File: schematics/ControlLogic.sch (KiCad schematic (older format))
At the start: 22 parts

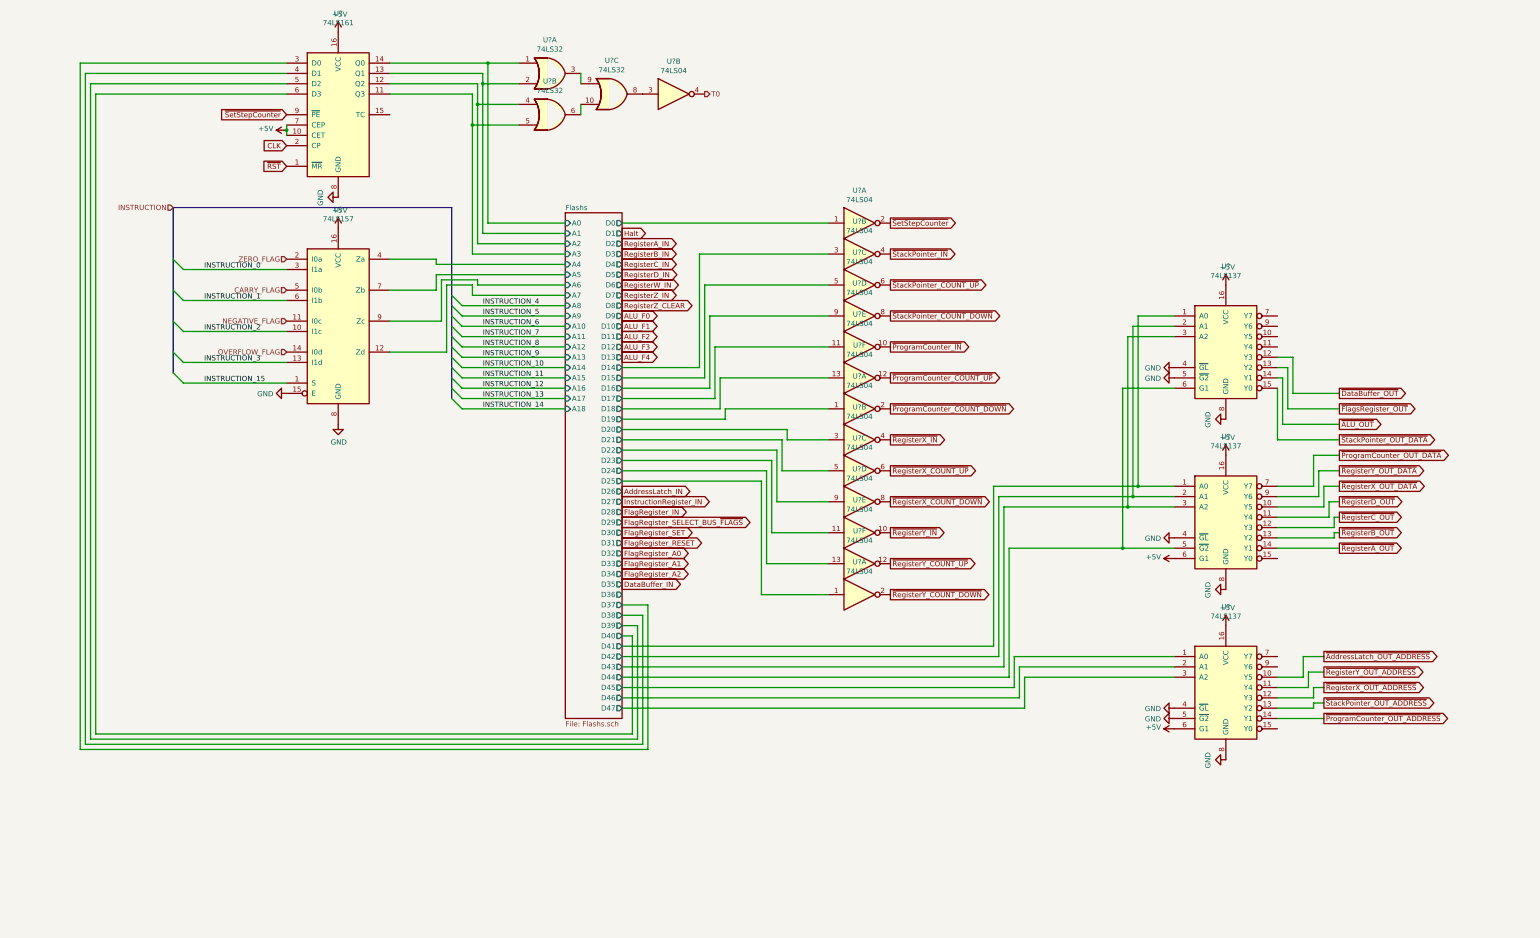
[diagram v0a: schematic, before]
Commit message: rearrange outputs of microcode eeproms
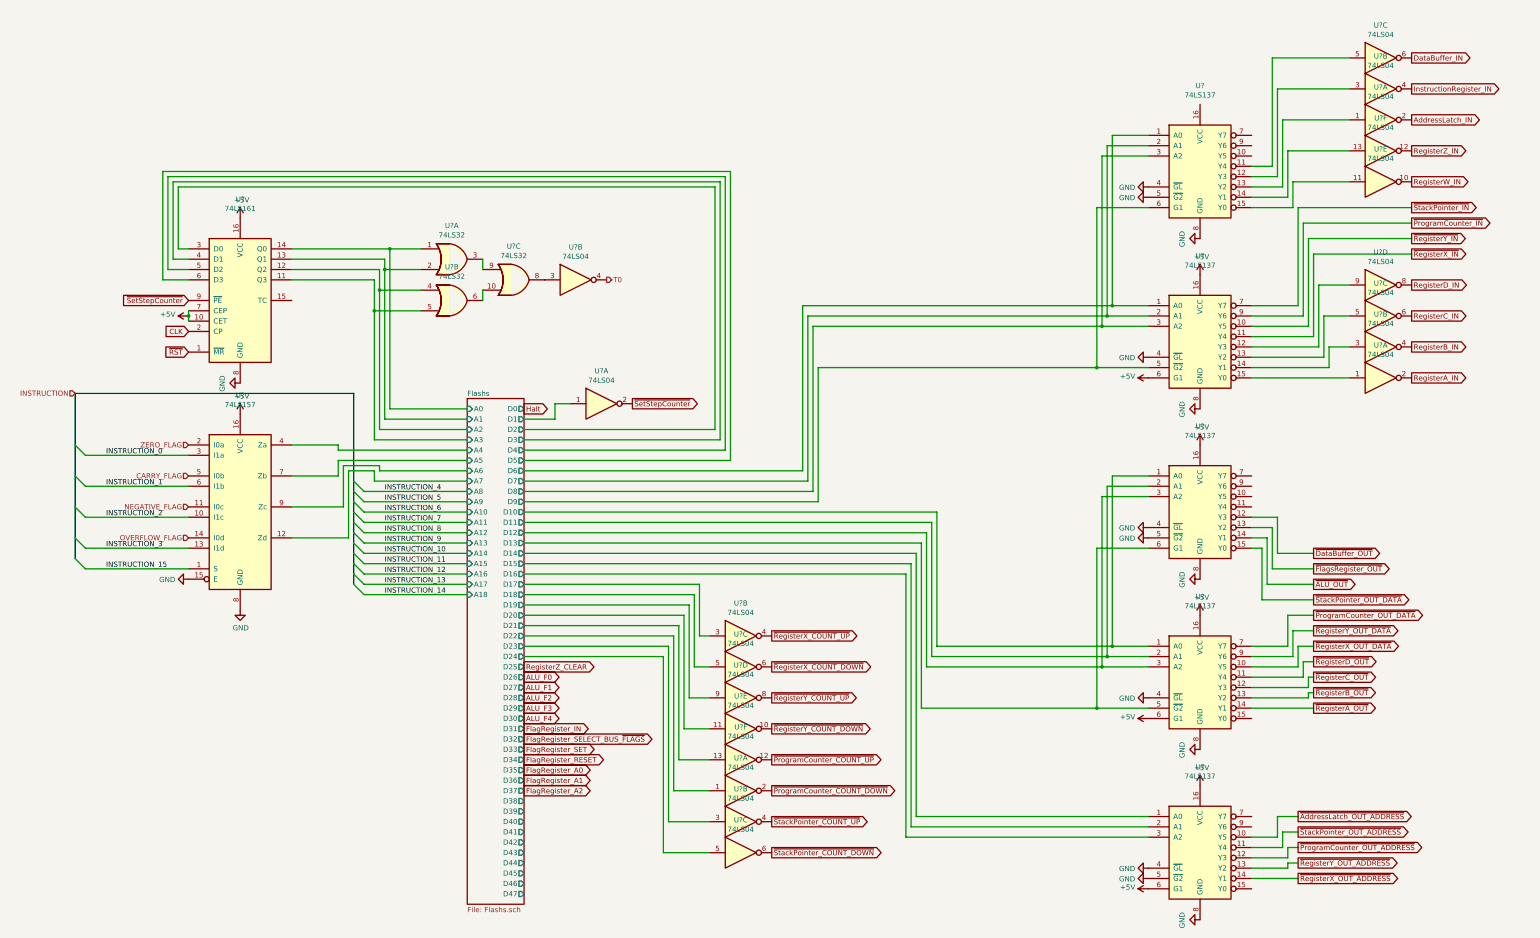
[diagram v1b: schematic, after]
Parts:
- removed U? (x4): 74LS04, symbol 74xx:74LS04
- added U? (x2): 74LS137, symbol 74xx:74LS137
- added U? (x9): 74LS04, symbol 74xx:74LS04
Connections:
- net +5V: now also U?.16 (VCC), U?.6 (G1)
- net AddressLatch_IN: now also U?.2
- net DataBuffer_IN: now also U?.6
- net Flashs/D14: now also U?.1 (A0); no longer U?.3
- net Flashs/D15: now also U?.2 (A1); no longer U?.5
- net Flashs/D16: now also U?.3 (A2); no longer U?.9
- net Flashs/D17: now also U?.3; no longer U?.11
- net Flashs/D18: now also U?.5; no longer U?.13
- net Flashs/D19: now also U?.9; no longer U?.1
- net Flashs/D20: now also U?.11; no longer U?.3
- net Flashs/D21: now also U?.13; no longer U?.5
- net Flashs/D22: now also U?.1
- net Flashs/D23: now also U?.3
- net Flashs/D24: now also U?.5
- net Flashs/D38: no longer U?.4 (D1)
- net Flashs/D39: no longer U?.5 (D2)
- net Flashs/D40: no longer U?.6 (D3)
- net Flashs/D41: no longer U?.1 (A0), U?.1 (A0)
- net Flashs/D42: no longer U?.2 (A1), U?.2 (A1)
- net Flashs/D43: no longer U?.3 (A2), U?.3 (A2)
- net Flashs/D44: no longer U?.5 (~G2), U?.6 (G1)
- net Flashs/D45: no longer U?.1 (A0)
- net Flashs/D46: no longer U?.2 (A1)
- net Flashs/D47: no longer U?.3 (A2)
- net GND: now also U?.4 (~GL), U?.4 (~GL), U?.5 (~G2), U?.8 (GND), U?.8 (GND)
- net InstructionRegister_IN: now also U?.4
- net RegisterA_IN: now also U?.2
- net RegisterB_IN: now also U?.4
- net RegisterC_IN: now also U?.6
- net RegisterD_IN: now also U?.8
- net RegisterW_IN: now also U?.10
- net RegisterZ_IN: now also U?.12
- net ~ProgramCounter_IN: now also U?.9 (Y6); no longer U?.10
- net ~ProgramCounter_OUT_ADDRESS: now also U?.12 (Y3); no longer U?.14 (Y1)
- net ~RegisterX_COUNT_DOWN: now also U?.6
- net ~RegisterX_COUNT_UP: now also U?.4; no longer U?.6
- net ~RegisterX_IN: now also U?.11 (Y4); no longer U?.4
- net ~RegisterX_OUT_ADDRESS: now also U?.14 (Y1); no longer U?.12 (Y3)
- net ~RegisterY_COUNT_DOWN: now also U?.10
- net ~RegisterY_COUNT_UP: now also U?.8
- net ~RegisterY_IN: now also U?.10 (Y5)
- net ~RegisterY_OUT_ADDRESS: now also U?.13 (Y2); no longer U?.11 (Y4)
- net ~StackPointer_COUNT_DOWN: now also U?.6; no longer U?.8
- net ~StackPointer_COUNT_UP: now also U?.4; no longer U?.6
- net ~StackPointer_IN: now also U?.7 (Y7); no longer U?.4
- net ~StackPointer_OUT_ADDRESS: now also U?.11 (Y4); no longer U?.13 (Y2)
- net Flashs/D0 renamed Flashs/D1
- net Flashs/D37 renamed Flashs/D2
- new net: U?.11 (Y4), U?.5
- new net: U?.12 (Y3), U?.3
- new net: U?.1, U?.13 (Y2)
- new net: U?.13, U?.14 (Y1)
- new net: U?.11, U?.15 (Y0)
- new net: U?.12 (Y3), U?.9
- new net: U?.13 (Y2), U?.5
- new net: U?.14 (Y1), U?.3
- new net: U?.1, U?.15 (Y0)
- new net Flashs/D10: U?.1 (A0), U?.1 (A0)
- new net Flashs/D11: U?.2 (A1), U?.2 (A1)
- new net Flashs/D12: U?.3 (A2), U?.3 (A2)
- new net Flashs/D13: U?.5 (~G2), U?.6 (G1)
- new net Flashs/D3: U?.4 (D1)
- new net Flashs/D4: U?.5 (D2)
- new net Flashs/D5: U?.6 (D3)
- new net Flashs/D6: U?.1 (A0), U?.1 (A0)
- new net Flashs/D7: U?.2 (A1), U?.2 (A1)
- new net Flashs/D8: U?.3 (A2), U?.3 (A2)
- new net Flashs/D9: U?.5 (~G2), U?.6 (G1)
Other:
- moved on the sheet: U?, U?A, U?B, U?C, U?D, U?E, U?F
